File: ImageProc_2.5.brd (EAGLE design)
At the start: 45.7 x 20.3 mm, 50 parts, among them J2 MOLEX_5034800600, U1 MIC5335-SPYMT, U11 ANTENNA-CHIP, U2 MIC5320-JGYML, U3 AT45DB321D, U4 ITG-3200, U6 ECS-2033, U7 ECS-160-8, U8 AT86RF231-ZU, U9 MN13822-L

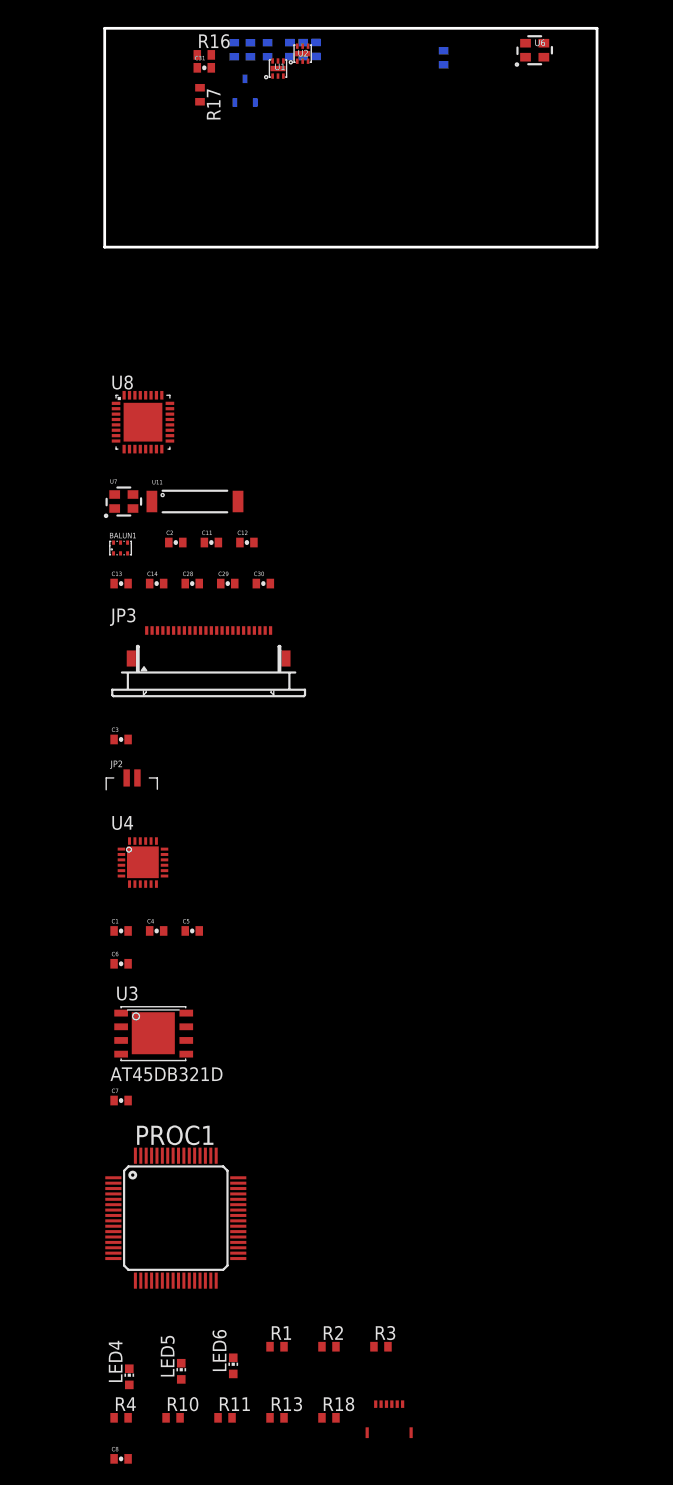
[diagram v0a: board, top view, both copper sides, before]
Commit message: Stopped commiting for a week. Oops.
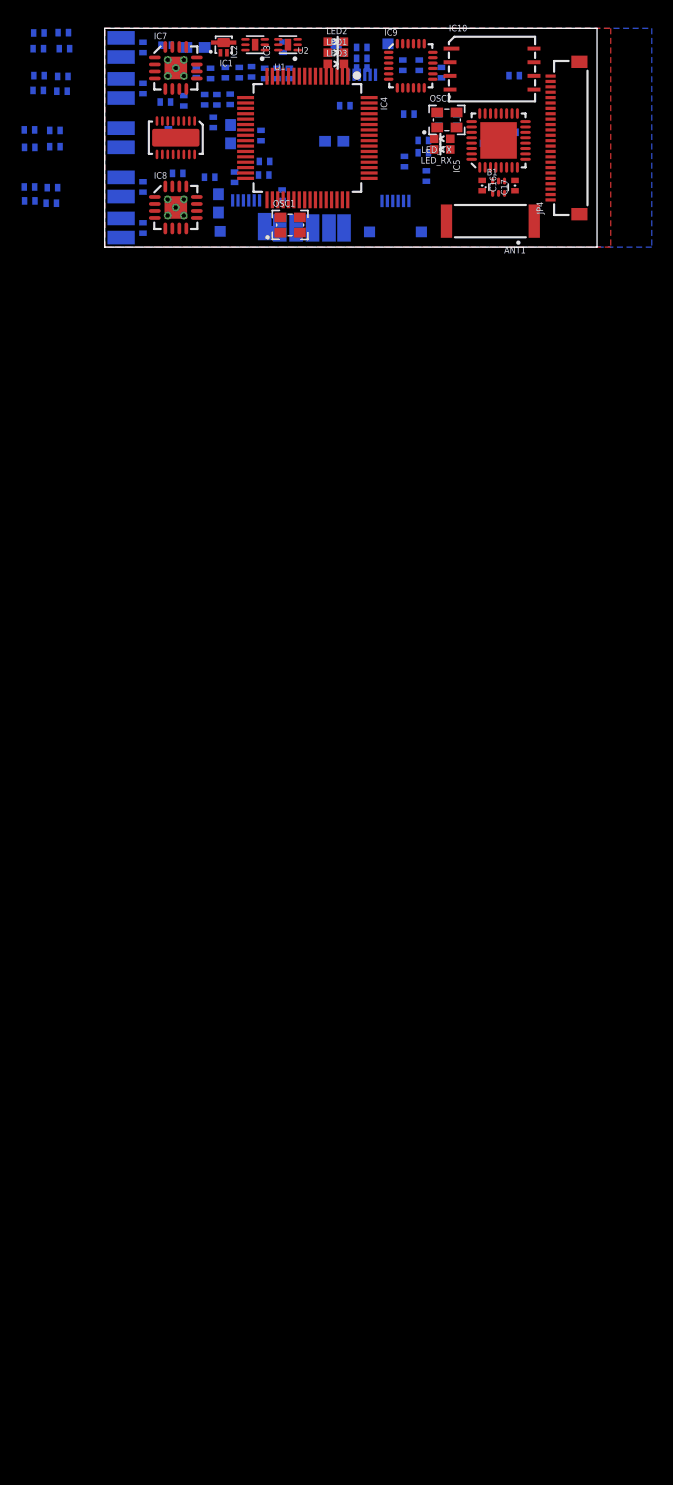
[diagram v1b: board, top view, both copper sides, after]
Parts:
- removed BALUN1: HHM1710D1, stan:BALUN
- removed J2: MOLEX_5034800600, stan:MOLEX_5034800600
- removed LED4: Yellow, led:CHIP-LED0603
- removed LED5: Green, led:CHIP-LED0603
- removed LED6: Red, led:CHIP-LED0603
- removed PROC1: DSPIC33FJ128MC706A, stan:TQFP64
- removed U1: MIC5335-SPYMT, stan:MLF-6
- removed U11: ANTENNA-CHIP, stan:ANTENNA-CHIP
- removed U2: MIC5320-JGYML, stan:MLF-6
- removed U3: AT45DB321D, stan:MLF(VDFN)-8
- removed U4: ITG-3200, stan:QFN-24
- removed U6: ECS-2033, stan:OSCILLATOR-SMD
- removed U7: ECS-160-8, stan:CRYSTAL-SMD
- removed U8: AT86RF231-ZU, stan:QFN-32
- removed U9: MN13822-L, stan:SOT-23-3
- added ANT1: ANT8030-2R4-01A, biomimetic:ANT8030-2R4-01A
- added B1: HHM1710D1, biomimetic:0603-BALUN
- added C10, C20, C22, C27, C36, C37, C39, C40, C9: 0.1uF, biomimetic:0402-CAP
- added C18, C19: 10pF, biomimetic:0402-CAP
- added C21: 1uF, biomimetic:0402-CAP
- added C32, C35: 2.2uF, biomimetic:0402-CAP
- added C33: 22uF, biomimetic:0603-CAP
- added C34: 10nF, biomimetic:0402-CAP
- added C38: 2.2nF, biomimetic:0402-CAP
- added IC1: XC61GC3002HR-G, biomimetic:USP-3
- added IC10: AT45DB642D-CNU, biomimetic:CASON-8
- added IC2: MIC5335-SPYMT, biomimetic:MLF-6
- added IC3: MIC5335-JGYMT, biomimetic:MLF-6
- added IC4: DSPIC33FJ128MC706A, biomimetic:TQFP-64
- added IC5: AT86RF233-ZU, biomimetic:VQFN-32QN2
- added IC6: LTC6088, biomimetic:DFN-16
- added IC7, IC8: DRV8833RTY, biomimetic:S-PWQFN-N16
- added IC9: MPU-6000, biomimetic:QFN-24
- added JP1: MOLEX_503480-0600, biomimetic:MOLEX_503480-0600
- added JP4: 51441-2493-C, biomimetic:MOLEX_52740-2490
- added L1: 4.7uH, biomimetic:0603
- added LED1: YELLOW, biomimetic:LED-0603
- added LED2, LED_RX: GREEN, biomimetic:LED-0603
- added LED3, LED_TX: RED, biomimetic:LED-0603
- added OSC1: ECS-2033-400, biomimetic:OSCILLATOR-SMD
- added OSC2: NX2520SA-16.000000MHZ, biomimetic:CRYSTAL-SMD
- added P1: BAT+, wirepad:SMD1,27-2,54
- added P10: MD2, wirepad:SMD1,27-2,54
- added P11: EXT1, wirepad:SMD1,27-2,54
- added P12: EXT2, wirepad:SMD1,27-2,54
- added P13: EXT3, wirepad:SMD1,27-2,54
- added P14: EXT4, wirepad:SMD1,27-2,54
- added P15: EXT5, wirepad:SMD1,27-2,54
- added P16: EXT6, wirepad:SMD1,27-2,54
- added P2: BAT-, wirepad:SMD1,27-2,54
- added P3: MA1, wirepad:SMD1,27-2,54
- added P4: MA2, wirepad:SMD1,27-2,54
- added P5: MB1, wirepad:SMD1,27-2,54
- added P6: MB2, wirepad:SMD1,27-2,54
- added P7: MC1, wirepad:SMD1,27-2,54
- added P8: MC2, wirepad:SMD1,27-2,54
- added P9: MD1, wirepad:SMD1,27-2,54
- added R12, R15, R21, R22, R25, R8: 15k, biomimetic:0402-RES
- added R14, R19, R20, R23, R24, R9: 47k, biomimetic:0402-RES
- added R26, R27, R28, R6, R7: 2.7k, biomimetic:0402-RES
- added R5: 4.7k, biomimetic:0402-RES
- C1: value 2.2nF -> 1uF; device SparkFun:0402-CAP -> biomimetic:0402-CAP
- C11, C12, C13, C24, C25, C26: value 1uF -> 0.1uF; device SparkFun:0402-CAP -> biomimetic:0402-CAP
- C14, C28: value 22pF -> 0.1uF; device SparkFun:0402-CAP -> biomimetic:0402-CAP
- C15: value 1uF -> 4.7uF; device SparkFun:0402-CAP -> biomimetic:0603-CAP
- C16, C17: value 1uF -> 22pF; device SparkFun:0402-CAP -> biomimetic:0402-CAP
- C2, C3, C31: device SparkFun:0402-CAP -> biomimetic:0402-CAP
- C23, C4, C5, C7: value 0.1uF -> 1uF; device SparkFun:0402-CAP -> biomimetic:0402-CAP
- C29: value 12pF -> 0.1uF; device SparkFun:0402-CAP -> biomimetic:0402-CAP
- C30: value 12pF -> 22uF; device SparkFun:0402-CAP -> biomimetic:0603-CAP
- C6: value 10nF -> 0.1uF; device SparkFun:0402-CAP -> biomimetic:0402-CAP
- C8: value 2.2uF -> 1uF; device SparkFun:0402-CAP -> biomimetic:0402-CAP
- JP2: value MPCS2PH -> MOLEX_503480-0600; device stan:MOLEX-PICO_CLASP_S2P -> biomimetic:MOLEX_503480-0600
- JP3: value 51441-2493-C -> MOLEX_503480-0600; device stan:MOLEX-52740-2490 -> biomimetic:MOLEX_503480-0600
- R1: value 4.7k -> 1k; device rcl:R0402 -> biomimetic:0402-RES
- R10: value 10k -> 47k; device rcl:R0402 -> biomimetic:0402-RES
- R11: value 470 -> 15k; device rcl:R0402 -> biomimetic:0402-RES
- R13: value 470 -> 47k; device rcl:R0402 -> biomimetic:0402-RES
- R16: value 27K -> 4.7k; device rcl:R0402 -> biomimetic:0402-RES
- R17: value 10K -> 15k; device rcl:R0402 -> biomimetic:0402-RES
- R18: value 470 -> 4.7k; device rcl:R0402 -> biomimetic:0402-RES
- R2: value 4.7k -> 2.7k; device rcl:R0402 -> biomimetic:0402-RES
- R3, R4: device rcl:R0402 -> biomimetic:0402-RES
- moved C8 129.4 mm to (13.6, 16.3), flipped to the bottom, turned to 270 degrees
- moved R10 129.2 mm to (-6.11, 19.9), flipped to the bottom
- moved R11 128.3 mm to (-6.16, 18.4), flipped to the bottom
- moved R13 126.6 mm to (-6.10, 15.9), flipped to the bottom, turned to 180 degrees
- moved R18 122.8 mm to (11.7, 13.7), flipped to the bottom, turned to 270 degrees
- moved R4 119.8 mm to (14.5, 10.4), flipped to the bottom, turned to 270 degrees
- moved R2 118.7 mm to (9.83, 16.1), flipped to the bottom, turned to 270 degrees
- moved R1 118.4 mm to (12.5, 16.2), flipped to the bottom, turned to 90 degrees
- moved R3 114.5 mm to (28.2, 12.4), flipped to the bottom
- moved C7 96.3 mm to (14.9, 16.1), flipped to the bottom, turned to 270 degrees
- moved C1 83.4 mm to (16.6, 18.6), flipped to the bottom, turned to 270 degrees
- moved C6 83.3 mm to (11.2, 16.2), flipped to the bottom, turned to 90 degrees
- moved C5 82.3 mm to (5.71, 18.7), flipped to the bottom
- moved C4 77.3 mm to (9.28, 13.7), flipped to the bottom, turned to 90 degrees
- moved C3 62.3 mm to (8.51, 16.2), flipped to the bottom, turned to 270 degrees
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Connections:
- removed net AN0: C31.2, PROC1.16, R16.2, R17.1
- removed net AN1: PROC1.15
- removed net AN10: PROC1.23
- removed net AN11: PROC1.24
- removed net AN3: PROC1.13
- removed net AN4: PROC1.12
- removed net AN5: PROC1.11
- removed net BAT+: C15.1, C24.1, JP2.1, R17.2, U1.1, U1.3, U1.4, U2.1, U2.3, U2.4, U9.2
- removed net INT1: PROC1.42, U4.12
- removed net INT2: PROC1.43, U9.1
- removed net INT3: PROC1.44
- removed net INT4: PROC1.45, U8.24
- removed net MCLR: J2.P5, PROC1.7, R10.1
- removed net OSC1: JP3.12, PROC1.39, U6.3
- removed net OSC2: PROC1.40
- removed net PWM1: PROC1.60
- removed net PWM1H: PROC1.61
- removed net PWM2: PROC1.62
- removed net PWM2H: PROC1.63
- removed net PWM3: PROC1.64
- removed net PWM3H: PROC1.1
- removed net PWM4: PROC1.2
- removed net PWM4H: PROC1.3
- removed net RB15: PROC1.30, U8.11
- removed net RC13: JP3.18, PROC1.47
- removed net RC14: JP3.17, PROC1.48
- removed net RD0: PROC1.46
- removed net RD1: PROC1.49
- removed net RD10: JP3.6
- removed net RD11: JP3.7
- removed net RD12: JP3.9
- removed net RD13: JP3.11
- removed net RD14: JP3.13
- removed net RD15: JP3.4
- removed net RD2: PROC1.50
- removed net RD3: PROC1.51
- removed net RD4: PROC1.52
- removed net RD5: PROC1.53
- removed net RD6: PROC1.54
- removed net RD7: PROC1.55
- removed net RD8: JP3.3
- removed net RD9: JP3.5
- removed net RF0: JP3.16, PROC1.58
- removed net RF1: JP3.8, PROC1.59
- removed net SCL2: PROC1.32, R4.1, U4.23
- removed net SDA2: PROC1.31, R3.1, U4.24
- removed net SS1: PROC1.14, U8.23
- removed net SS2: PROC1.8, U3.4
- removed net VCC: C17.1, C3.2, JP3.14, JP3.21, U2.6
- removed net VDD: C12.1, C2.1, C23.1, C25.1, C4.1, C6.1, C7.1, J2.P4, PROC1.10, PROC1.19, PROC1.26, PROC1.38, PROC1.57, R1.2, R10.2, R2.2, R3.2, R4.2, U1.6, U3.3, U3.5, U3.6, U4.13, U4.8, U6.4, U8.15, U8.28, U8.8
- removed net VEE: C16.1, JP3.15, U2.5
- removed net VPP: C26.1, U1.5
- new net !RESET: IC10.3, IC4.7, IC5.8, JP1.1, R3.1
- new net !SS1: IC4.14, IC5.23
- new net !SS2_1: IC10.4, IC4.8
- new net !SS2_2: IC4.40, IC9.8
- new net 1.8V: C8.1, IC3.5, JP4.15
- new net 2.5V: C2.1, C36.2, IC3.6, JP4.14, JP4.21
- new net 3.0V: C7.1, IC2.5
- new net 3.3V: C1.1, C11.1, C12.1, C13.1, C14.1, C21.1, C23.1, C37.1, C40.1, C9.1, IC10.5, IC10.6, IC2.6, IC4.10, IC4.26, IC4.38, IC4.57, IC5.15, IC5.28, IC9.13, JP1.2, JP3.1, L1.2, OSC1.4, R3.2, R4.2, R5.2
- new net 40MHZ: IC4.39, JP4.12, OSC1.3
- new net BATT_LEVEL: C6.1, IC4.16, R1.1, R2.2
- new net CAM_D0: IC4.46, JP4.6
- new net CAM_D1: IC4.49, JP4.4
- new net CAM_D2: IC4.50, JP4.3
- new net CAM_D3: IC4.51, JP4.5
- new net CAM_D4: IC4.52, JP4.7
- new net CAM_D5: IC4.53, JP4.9
- new net CAM_D6: IC4.54, JP4.11
- new net CAM_D7: IC4.55, JP4.13
- new net CAM_HREF: IC4.58, IC9.11, JP4.16
- new net CAM_PCLK: IC4.59, JP4.8
- new net CAM_PWDN: IC4.48, JP4.17
- new net CAM_VSYNC: IC4.47, JP4.18
- new net EXT1: IC4.15, P11.1
- new net EXT2: IC4.13, P12.1
- new net EXT3: IC4.12, P13.1
- new net EXT4: IC4.11, P14.1
- new net EXT5: IC4.42, P15.1
- new net EXT6: IC4.44, P16.1
- new net GN_LED: IC4.28, LED2.A
- new net LOWBATT_IRQ: IC1.2, IC4.43
- new net MOTOR_A_BEMF: IC4.21, IC6.1, R8.2
- new net MOTOR_A_IN1: IC4.61, IC7.14
- new net MOTOR_A_IN2: IC4.60, IC7.13
- new net MOTOR_A_OUT1: C24.1, IC7.16, P3.1, R9.1
- new net MOTOR_A_OUT2: C24.2, IC7.2, P4.1, R10.1
- new net MOTOR_B_BEMF: IC4.22, IC6.7, R12.2
- new net MOTOR_B_IN1: IC4.63, IC7.7
- new net MOTOR_B_IN2: IC4.62, IC7.8
- new net MOTOR_B_OUT1: C25.1, IC7.5, P5.1, R13.1
- new net MOTOR_B_OUT2: C25.2, IC7.3, P6.1, R14.1
- new net MOTOR_C_BEMF: IC4.23, IC6.10, R17.2
- new net MOTOR_C_IN1: IC4.1, IC8.14
- new net MOTOR_C_IN2: IC4.64, IC8.13
- new net MOTOR_C_OUT1: C27.1, IC8.16, P7.1, R19.1
- new net MOTOR_C_OUT2: C27.2, IC8.2, P8.1, R20.1
- new net MOTOR_D_BEMF: IC4.24, IC6.16, R22.2
- new net MOTOR_D_IN1: IC4.3, IC8.7
- new net MOTOR_D_IN2: IC4.2, IC8.8
- new net MOTOR_D_OUT1: C28.1, IC8.5, P9.1, R23.1
- new net MOTOR_D_OUT2: C28.2, IC8.3, P10.1, R24.1
- new net N$1: C22.2, IC5.13, IC5.14
- new net N$11: LED_RX.C, R7.1
- new net N$21: C10.1, IC4.19, L1.1
- new net N$24: IC6.11, R17.1, R19.2
- new net N$3: C20.2, IC5.29
- new net N$31: IC6.3, R10.2, R11.2
- new net N$32: C39.2, IC9.10
- new net N$6: C16.1, IC5.4
- new net N$7: C17.2, IC5.5
- new net N$8: C19.1, IC5.25, OSC2.3
- new net N$9: C18.1, IC5.26, OSC2.1
- new net PGC: IC4.17, JP1.5
- new net PGD: IC4.18, JP1.4
- new net RADIO_IRQ: IC4.45, IC5.24
- new net RADIO_SLP_TR: IC4.30, IC5.11
- new net RD_LED: IC4.27, LED3.A
- new net U2RX: IC4.31, JP2.6
- new net U2TX: IC4.32, JP2.4
- new net V_BATT: C29.1, C3.1, C30.1, C31.1, C33.1, C34.1, C4.2, C5.2, IC1.3, IC2.1, IC2.3, IC2.4, IC3.1, IC3.3, IC3.4, IC6.4, IC7.10, IC7.15, IC8.10, IC8.15, JP2.1, JP2.2, P1.1, R1.2, R16.2
- new net V_REF: C26.1, R11.1, R15.1, R16.1, R18.2, R21.1, R25.1
- new net YW_LED: IC4.29, LED1.A
- net GND: now also B1.2, B1.5, C1.2, C10.2, C14.2, C18.2, C19.2, C20.1, C21.2, C22.1, C3.2, C32.2, C33.2, C35.2, C36.1, C37.2, C38.1, C39.1, C4.1, C40.2, C5.1, C9.2, IC1.1, IC10.7, IC2.2, IC2.EPAD, IC3.2, IC3.EPAD, IC4.20, IC4.25, IC4.41, IC4.9, IC5.12, IC5.16, IC5.18, IC5.21, IC5.27, IC5.3, IC5.30, IC5.31, IC5.32, IC5.6, IC5.7, IC5.PAD, IC6.13, IC6.PAD, IC7.1, IC7.11, IC7.4, IC7.PPAD, IC8.1, IC8.11, IC8.4, IC8.PPAD, IC9.1, IC9.18, JP1.3, JP2.3, JP2.5, JP3.2, JP3.4, JP3.6, JP4.10, JP4.19, JP4.23, OSC1.2, OSC2.2, OSC2.4, P2.1, R18.1, R2.1, R26.2, R27.2, R28.2, R6.2, R7.2; no longer BALUN1.2, BALUN1.5, BALUN1.6, C1.1, C16.2, C17.2, C24.2, C25.2, C3.1, C31.1, C4.2, C5.2, J2.P3, JP2.2, JP3.10, JP3.19, JP3.23, PROC1.20, PROC1.25, PROC1.41, PROC1.9, R11.2, R13.2, R16.1, R18.2, U1.2, U2.2, U3.7, U4.1, U4.11, U4.18, U4.9, U6.2, U7.2, U7.4, U8.12, U8.16, U8.18, U8.21, U8.27, U8.3, U8.30, U8.31, U8.32, U8.6, U8.7, U8.P$1, U9.3
- net N$10: now also B1.3, C17.1; no longer BALUN1.4, C14.1
- net N$12: now also B1.4, C16.2; no longer BALUN1.3, C28.1
- net N$13: now also IC5.1, LED_RX.A; no longer C14.2, U8.4
- net N$14: now also IC5.10, LED_TX.A; no longer C28.2, U8.5
- net N$15: now also LED1.C, R26.1; no longer BALUN1.1, U11.SIG
- net N$16: now also LED2.C, R27.1; no longer C30.1, U7.3, U8.25
- net N$17: now also LED3.C, R28.1; no longer C29.1, U7.1, U8.26
- net N$18: now also C32.1, IC7.12; no longer C1.2, U4.20
- net N$19: now also C34.2, IC8.9; no longer C5.1, U4.10
- net N$2: now also C31.2, IC7.9; no longer J2.P6, PROC1.21
- net N$20: now also C35.1, IC8.12; no longer LED4.C, R11.1
- net N$22: now also IC6.6, R12.1, R13.2; no longer LED4.A, PROC1.29
- net N$23: now also IC6.5, R14.2, R15.2; no longer J2.P1, PROC1.17
- net N$25: now also IC6.12, R20.2, R21.2; no longer J2.P2, PROC1.18
- net N$26: now also IC6.15, R22.1, R23.2; no longer LED5.C, R13.1
- net N$27: now also IC6.14, R24.2, R25.2; no longer LED6.C, R18.1
- net N$28: now also C15.1, IC4.56; no longer LED5.A, PROC1.28
- net N$29: now also C38.2, IC9.20; no longer LED6.A, PROC1.27
- net N$30: now also IC6.2, R8.1, R9.2; no longer C8.1, PROC1.56
- net N$4: now also ANT1.A, B1.1; no longer C11.1, U8.29
- net N$5: now also LED_TX.C, R6.1; no longer C13.1, U8.13, U8.14
- net SCK1: now also IC4.35, IC5.19; no longer PROC1.35, U8.19
- net SCK2: now also IC10.2, IC4.4, IC9.23; no longer PROC1.4, U3.2
- net SCL1: now also IC4.36, JP3.3, JP4.20, R4.1; no longer JP3.20, PROC1.37, R1.1
- net SDA1: now also IC4.37, JP3.5, JP4.22, R5.1; no longer JP3.22, PROC1.36, R2.1
- net SDI1: now also IC4.34, IC5.20; no longer PROC1.34, U8.20
- net SDI2: now also IC10.8, IC4.5, IC9.9; no longer PROC1.5, U3.8
- net SDO1: now also IC4.33, IC5.22; no longer PROC1.33, U8.22
- net SDO2: now also IC10.1, IC4.6, IC9.24; no longer PROC1.6, U3.1
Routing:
- added copper zone on layer 3, net 3.3V
- added copper zone on layer 1, net GND
- added copper zone on layer 16, net GND
- added copper zone on layer 2, net GND
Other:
- board text removed: "GYRO"
- board text removed: "I2C1"
- board text removed: "I2C2"
- board text removed: "ImageProc 2.4"
- board text removed: "LED"
- board text removed: "RADIO"
- board text removed: "UC Berkeley"
- board text removed: "WII"
- board text removed: "XL"

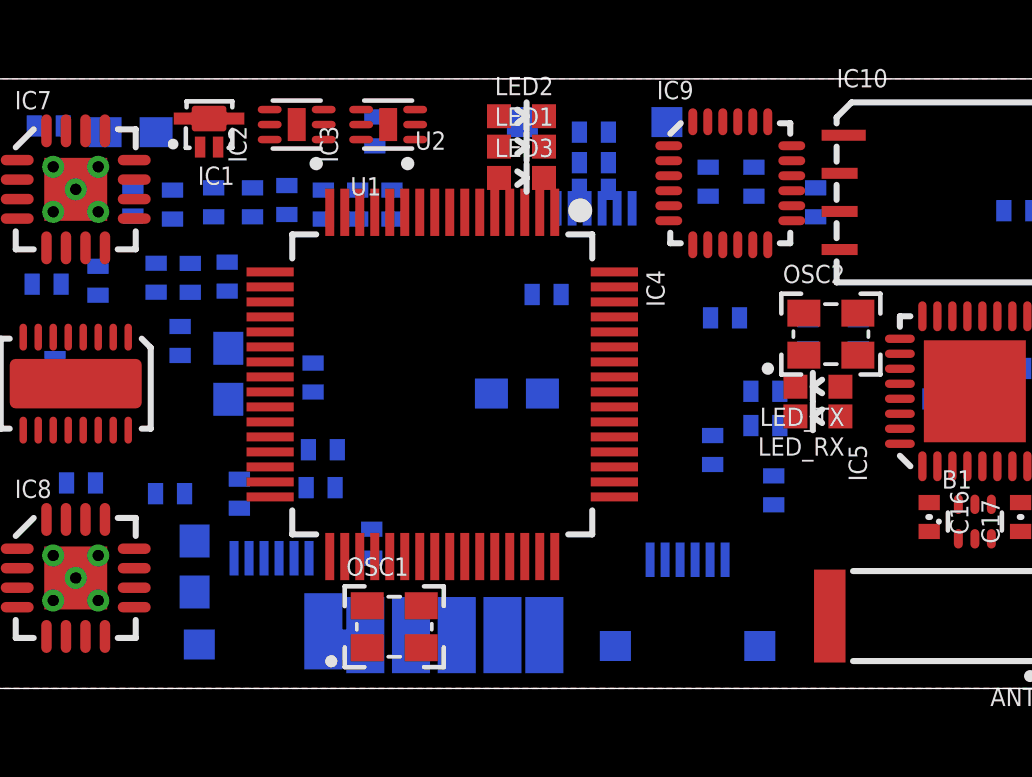
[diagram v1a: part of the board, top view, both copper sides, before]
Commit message: Before work 6/30
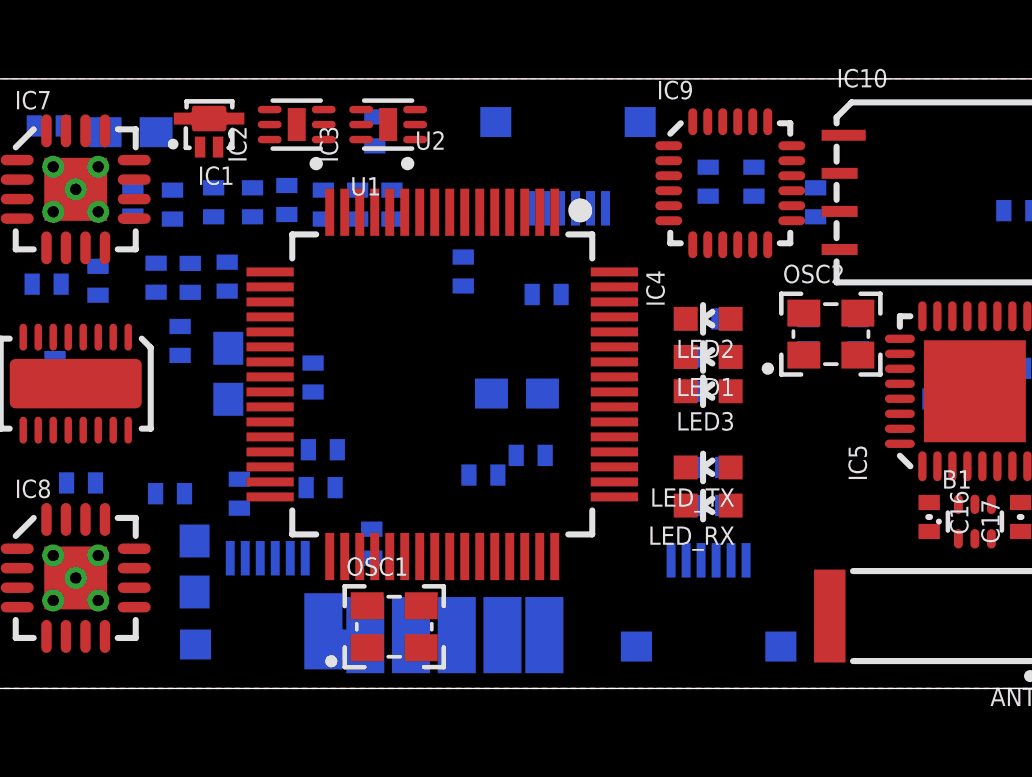
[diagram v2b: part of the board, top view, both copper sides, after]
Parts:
- moved C9 9.69 mm to (20.2, 7.11), turned to 0 degrees
- moved LED3 9.45 mm to (27.7, 9.91), turned to 90 degrees
- moved LED1 9.37 mm to (27.7, 11.0), turned to 90 degrees
- moved LED2 9.19 mm to (27.7, 12.3), turned to 90 degrees
- moved R3 8.86 mm to (19.5, 13.9), turned to 270 degrees
- moved R28 7.80 mm to (27.8, 9.91)
- moved R26 7.58 mm to (27.8, 11.0)
- moved R27 7.23 mm to (27.6, 12.3)
- moved C14 6.07 mm to (21.8, 7.77), turned to 0 degrees
- moved LED_RX 4.71 mm to (27.7, 6.10)
- moved LED_TX 4.54 mm to (27.7, 7.37)
- moved R7 3.28 mm to (27.7, 6.10), turned to 180 degrees
- moved R6 3.18 mm to (27.7, 7.37), turned to 180 degrees
- moved JP3 0.89 mm to (23.0, 17.7)
- moved JP1 0.70 mm to (27.7, 2.55)
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
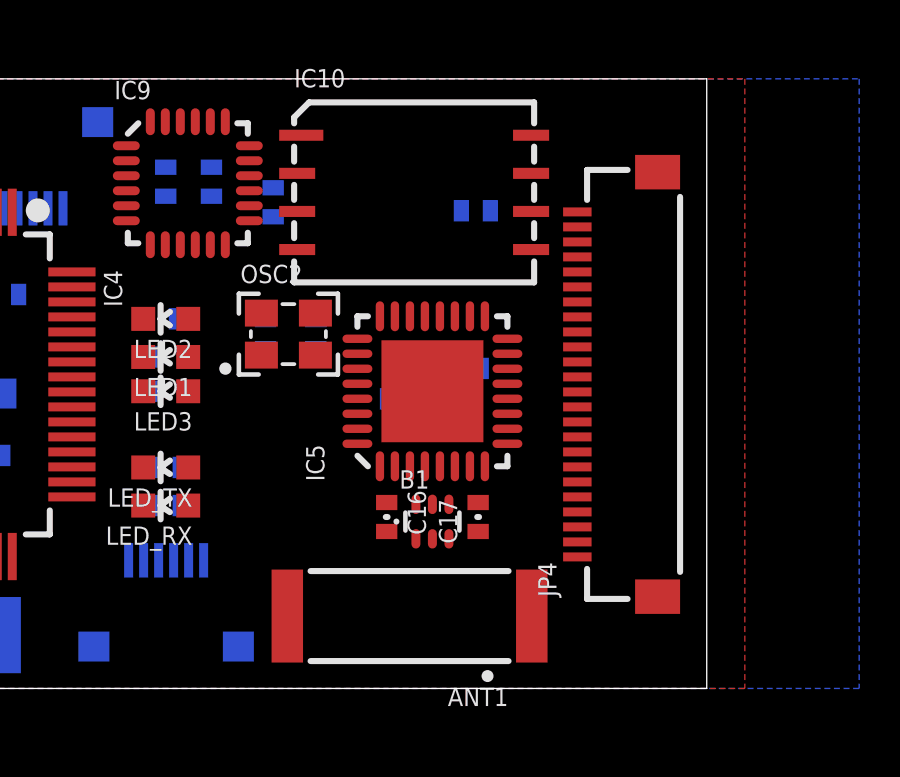
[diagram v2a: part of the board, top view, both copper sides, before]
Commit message: Work 6/30
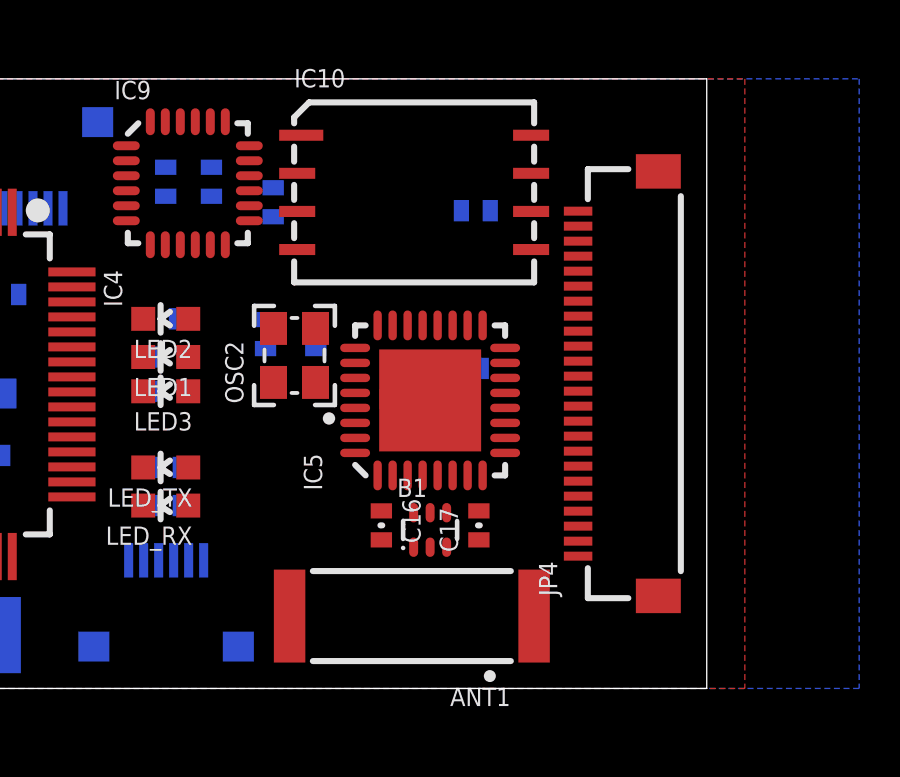
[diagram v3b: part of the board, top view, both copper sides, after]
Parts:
- moved OSC2 0.74 mm to (32.0, 11.1), turned to 90 degrees
- moved C16 0.33 mm to (34.9, 5.44)
- moved IC5 0.31 mm to (36.5, 9.60)
- moved B1 0.29 mm to (36.5, 5.28)
- moved C17 0.28 mm to (38.1, 5.44)
- moved ANT1 0.08 mm to (35.9, 2.41)
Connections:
- net 3.3V: now also C29.1, IC6.4
- net V_BATT: no longer C29.1, IC6.4
